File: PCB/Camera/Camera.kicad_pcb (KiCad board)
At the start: 2 copper layers, 85.5 x 66 mm, 3 parts, among them U4 ESP32-WROVER-E

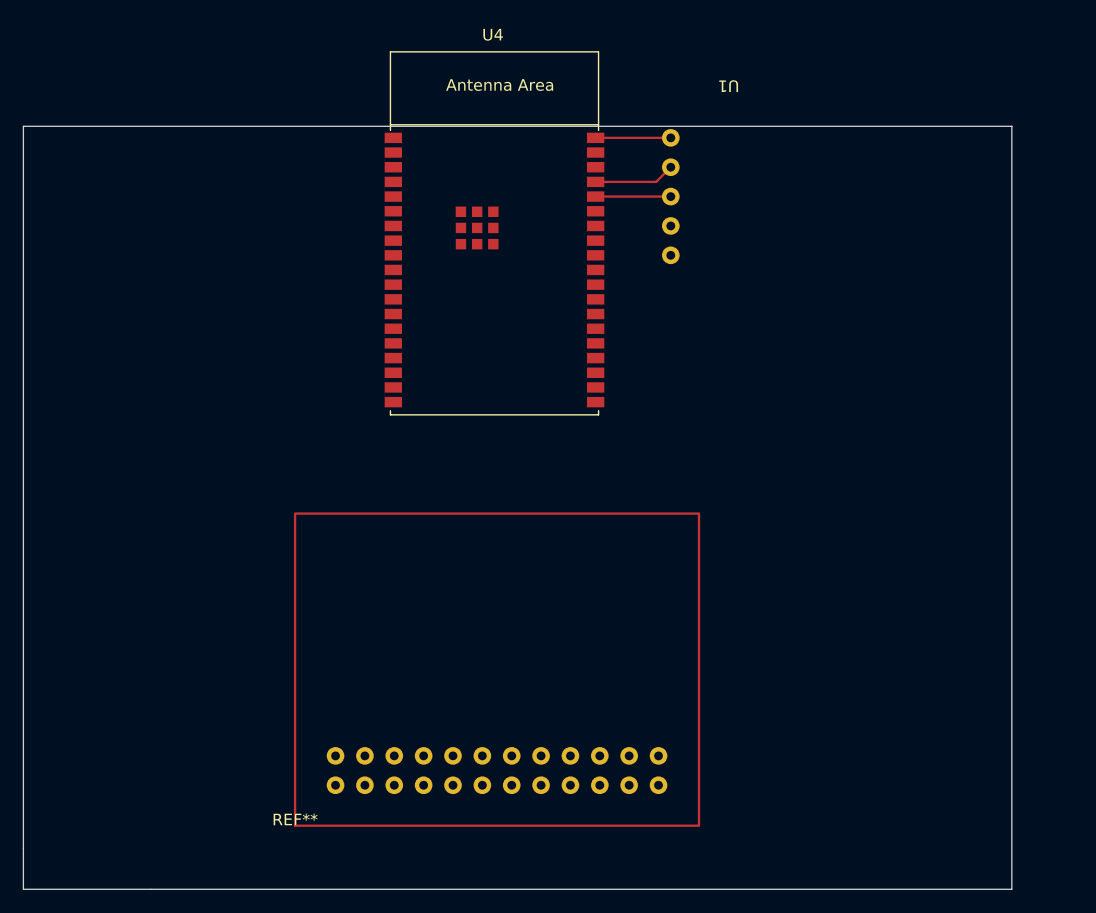
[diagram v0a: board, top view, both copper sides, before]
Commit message: PCB changes
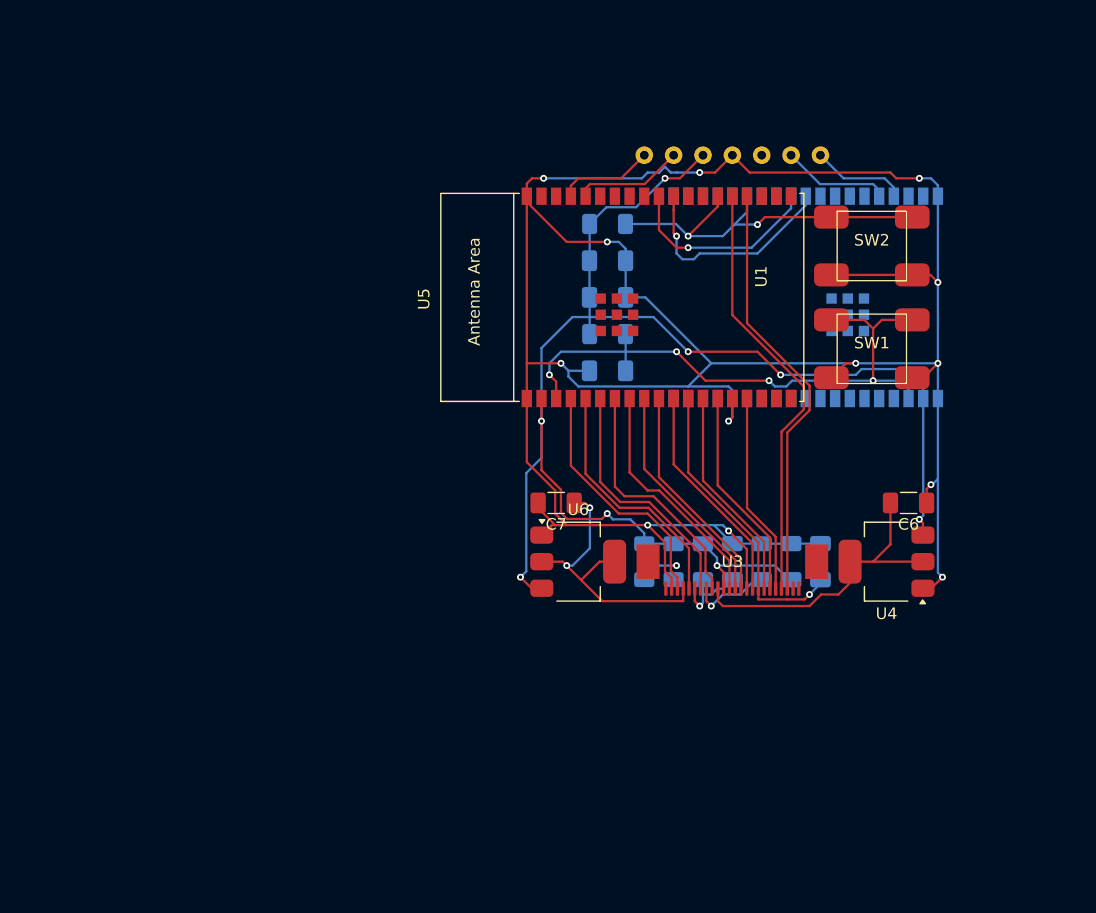
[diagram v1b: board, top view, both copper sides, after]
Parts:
- removed REF**: Camera_Interface, Camera_Components:Camera_Interface
- added C1: 0.1 uF, Capacitor_SMD:C_1206_3216Metric_Pad1.33x1.80mm_HandSolder, B.Cu at (176.5, 57.1)
- added C2: 15 pF, Capacitor_SMD:C_1206_3216Metric_Pad1.33x1.80mm_HandSolder, B.Cu at (194.9, 73.7)
- added C3: 0.1 uF, Capacitor_SMD:C_1206_3216Metric_Pad1.33x1.80mm_HandSolder, B.Cu at (187.3, 73.7)
- added C4: 0.1 uF, Capacitor_SMD:C_1206_3216Metric_Pad1.33x1.80mm_HandSolder, B.Cu at (192.4, 73.7)
- added C5: 10 uF, Capacitor_SMD:C_1206_3216Metric_Pad1.33x1.80mm_HandSolder, B.Cu at (176.5, 47.6)
- added C6: 22 uF, Capacitor_SMD:C_1206_3216Metric_Pad1.33x1.80mm_HandSolder, F.Cu at (202.6, 68.6)
- added C7: 22 uF, Capacitor_SMD:C_1206_3216Metric_Pad1.33x1.80mm_HandSolder, F.Cu at (172.1, 68.6)
- added C8: 0.1 uF, Capacitor_SMD:C_1206_3216Metric_Pad1.33x1.80mm_HandSolder, B.Cu at (176.5, 50.8)
- added R1: 10K, Resistor_SMD:R_1206_3216Metric_Pad1.30x1.75mm_HandSolder, B.Cu at (176.5, 54.0)
- added R2: 10K, Resistor_SMD:R_1206_3216Metric_Pad1.30x1.75mm_HandSolder, B.Cu at (176.5, 44.5)
- added R3: 1K, Resistor_SMD:R_1206_3216Metric_Pad1.30x1.75mm_HandSolder, B.Cu at (189.9, 73.7)
- added R4: 4.7K, Resistor_SMD:R_1206_3216Metric_Pad1.30x1.75mm_HandSolder, B.Cu at (184.8, 73.7)
- added R5: 4.7K, Resistor_SMD:R_1206_3216Metric_Pad1.30x1.75mm_HandSolder, B.Cu at (179.7, 73.7)
- added R6: 4.7K, Resistor_SMD:R_1206_3216Metric_Pad1.30x1.75mm_HandSolder, B.Cu at (182.2, 73.7)
- added SW1: SW_Push, Camera_Components:6x6x4.3 SMD button, F.Cu at (199.4, 55.2)
- added SW2: SW_Push, Camera_Components:6x6x4.3 SMD button, F.Cu at (199.4, 46.4)
- added U2: ~, PCM_Espressif:ESP32-WROVER-E, B.Cu at (196.8, 50.8)
- added U3: ~, Camera_Components:24-pin-FPC-0.5mm, F.Cu at (187.3, 73.7)
- added U5: ~, PCM_Espressif:ESP32-WROVER-E, F.Cu at (177.8, 50.8)
- added U6: AMS1117-2.85, Package_TO_SOT_SMD:SOT-223-3_TabPin2, F.Cu at (174.0, 73.7)
- U4: value ESP32-WROVER-E -> AMS1117-1.2; footprint PCM_Espressif:ESP32-WROVER-E -> Package_TO_SOT_SMD:SOT-223-3_TabPin2
- moved U4 44.2 mm to (200.7, 73.7), turned to 180 degrees
- moved U1 6.51 mm to (187.3, 38.5), turned to 90 degrees
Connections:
- U1 pad 1: GNDREF -> /B_TX
- U1 pad 2: /FLASH TX -> /B_RX
- U1 pad 3: /FLASH RX -> unconnected-(U1-5V-Pad3)
- U1 pad 4: /3.3V -> GNDREF
- U1 pad 5: unconnected-(U1-5V-Pad5) -> /3.3V
- U4 pad 2: /3.3V -> /1.2V
- U4 pad 3: /EN -> /3.3V
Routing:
- net GNDREF: track 6.50 -> 236.6 mm, vias 0 -> 13
- net /3.3V: track 0.00 -> 131.3 mm, vias 0 -> 8
- net /B_EN: track 0.00 -> 52.7 mm, vias 0 -> 4
- net /CAM_DATA3: track 0.00 -> 37.3 mm
- net /CAM_DATA4: track 0.00 -> 37.0 mm
- net /B_IO0: track 0.00 -> 33.3 mm, vias 0 -> 2
- net /1.2V: track 0.00 -> 27.4 mm
- net /CAM_PCLK: track 0.00 -> 26.2 mm, vias 0 -> 1
- net /2.8V: track 0.00 -> 25.9 mm, vias 0 -> 2
- net /CAM_SIOD: track 0.00 -> 25.5 mm, vias 0 -> 1
- net /CAM_SIOC: track 0.00 -> 21.6 mm
- net /CAM_VSYNC: track 0.00 -> 21.5 mm
- net /CAM_HREF: track 0.00 -> 21.4 mm
- net /CAM_DATA9: track 0.00 -> 20.6 mm
- net /CAM_XCLK: track 0.00 -> 19.7 mm
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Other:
- board outline removed

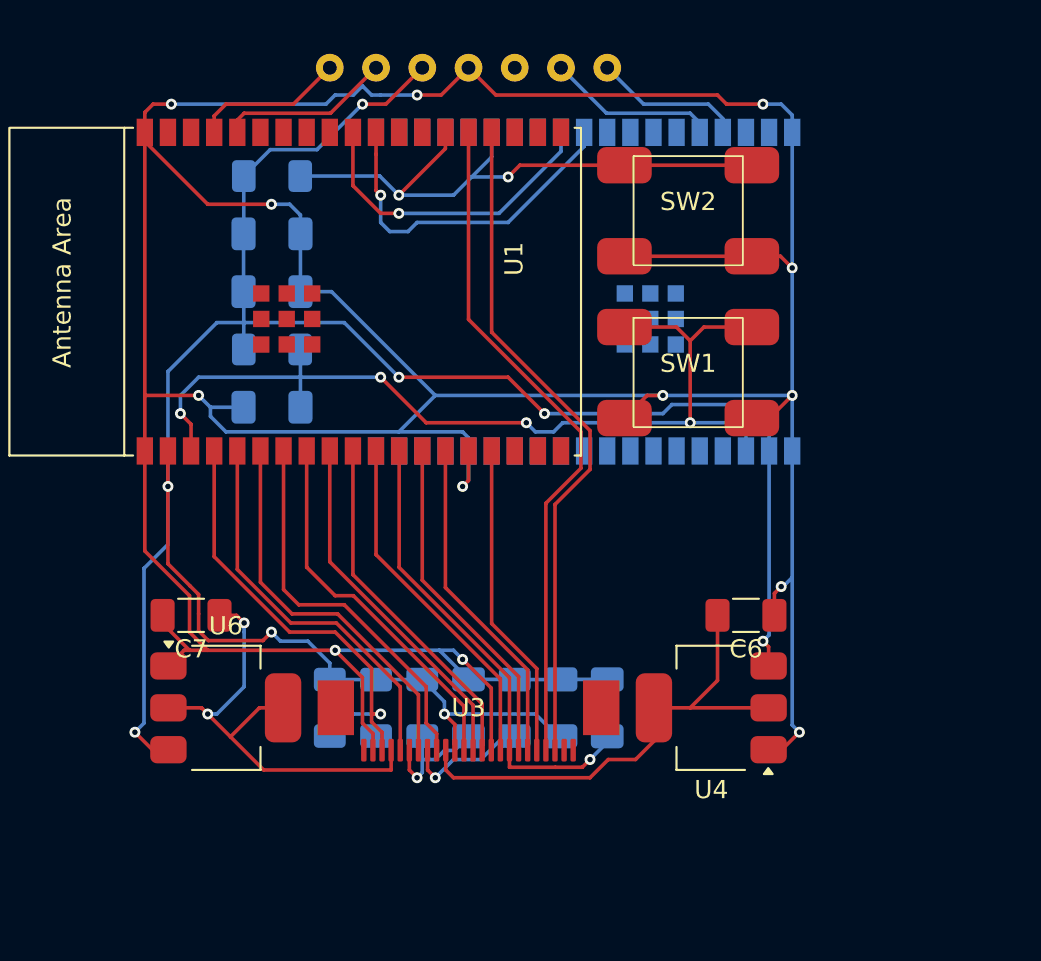
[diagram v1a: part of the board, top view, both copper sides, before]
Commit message: PCB changes
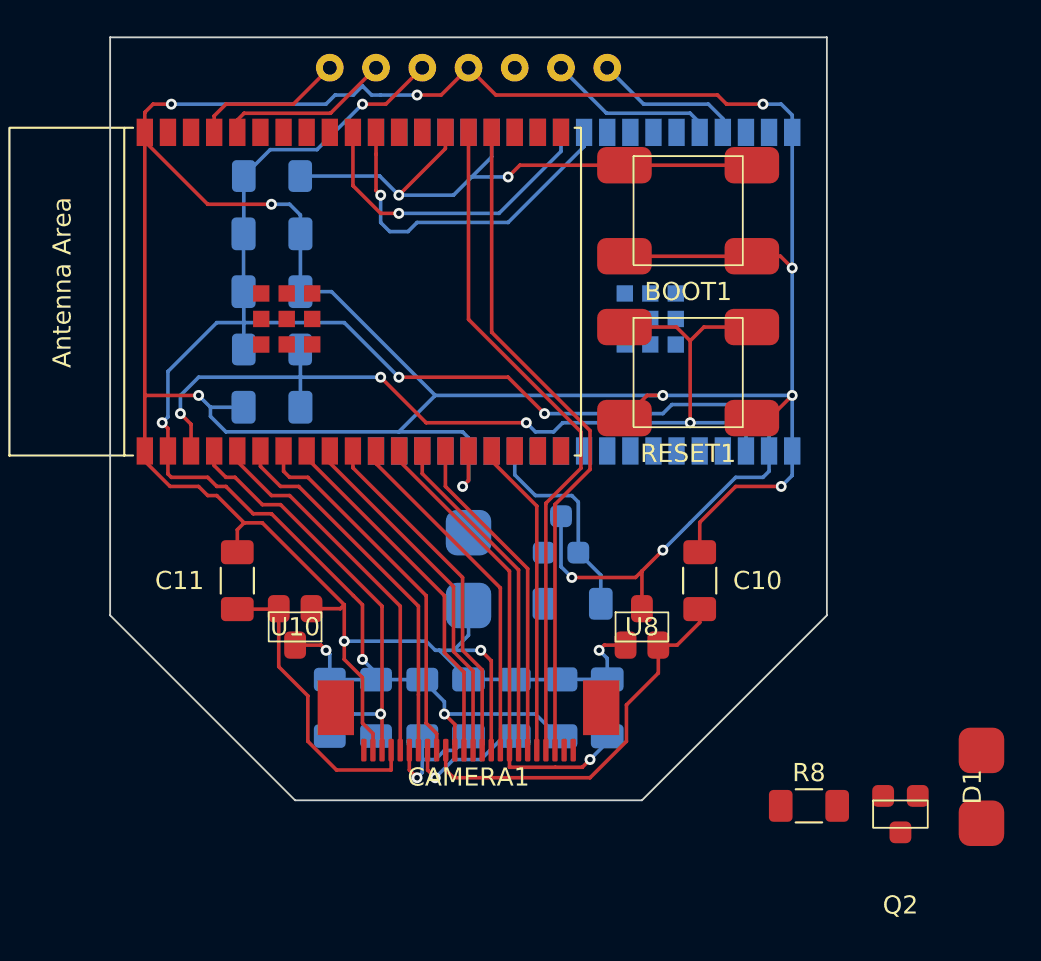
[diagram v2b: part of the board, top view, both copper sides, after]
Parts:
- removed C6, C7: 22 uF, Capacitor_SMD:C_1206_3216Metric_Pad1.33x1.80mm_HandSolder
- removed U4: AMS1117-1.2, Package_TO_SOT_SMD:SOT-223-3_TabPin2
- removed U6: AMS1117-2.85, Package_TO_SOT_SMD:SOT-223-3_TabPin2
- added C10: 1 uF, Capacitor_SMD:C_1206_3216Metric_Pad1.33x1.80mm_HandSolder, F.Cu at (200.0, 66.7)
- added C11: 1 uF, Capacitor_SMD:C_1206_3216Metric_Pad1.33x1.80mm_HandSolder, F.Cu at (174.6, 66.7)
- added D1: LED, Camera_Components:vibration motor, F.Cu at (215.5, 78.0)
- added Q1: S8050, Camera_Components:transistor, B.Cu at (192.4, 64.1)
- added Q2: S8050, Camera_Components:transistor, F.Cu at (211.1, 79.5)
- added R7: 4.7K, Resistor_SMD:R_1206_3216Metric_Pad1.30x1.75mm_HandSolder, B.Cu at (193.0, 67.9)
- added R8: 4.7K, Resistor_SMD:R_1206_3216Metric_Pad1.30x1.75mm_HandSolder, F.Cu at (206.0, 79.0)
- added U10: ~, Camera_Components:XC6206, F.Cu at (177.8, 69.2)
- added U7: ~, Camera_Components:vibration motor, B.Cu at (187.3, 66.0)
- added U8: ~, Camera_Components:XC6206, F.Cu at (196.8, 69.2)
- renumbered SW2 to BOOT1, U3 to CAMERA1, SW1 to RESET1
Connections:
- U2 pad 13: unconnected-(U2-IO14-Pad13) -> /V_CTRL
- U2 pad 8: unconnected-(U2-IO32-Pad8) -> /LED_CTRL
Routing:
- net /V_CTRL: track 0.00 -> 11.5 mm
- net /2.8V: track 25.9 -> 16.5 mm, vias 2 -> 0
- net GNDREF: track 236.6 -> 228.5 mm
- net /3.3V: track 131.3 -> 124.1 mm, vias 8 -> 9
- net /1.2V: track 27.4 -> 21.6 mm
- net /CAM_SIOD: track 25.5 -> 24.5 mm
- net /CAM_VSYNC: track 21.5 -> 20.6 mm
- net /CAM_HREF: track 21.4 -> 20.5 mm
- net /CAM_SIOC: track 21.6 -> 20.7 mm
- net /CAM_DATA9: track 20.6 -> 20.0 mm
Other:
- board outline added: 39.4 x 41.9 mm
